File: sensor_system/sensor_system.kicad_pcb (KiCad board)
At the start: 2 copper layers, 52 parts, among them J1 Magnetic connector, J2 Solar_panels, Q1 SBC817, Q2 MJD45H11, SW1 SW_DPDT_x2, U1 TLC555xD, U2 XC6206PxxxMR, U3 MCP73833, U4 module_bme280_alt, U5 ESP32-DEVKIT-V1, U7 TPS63002

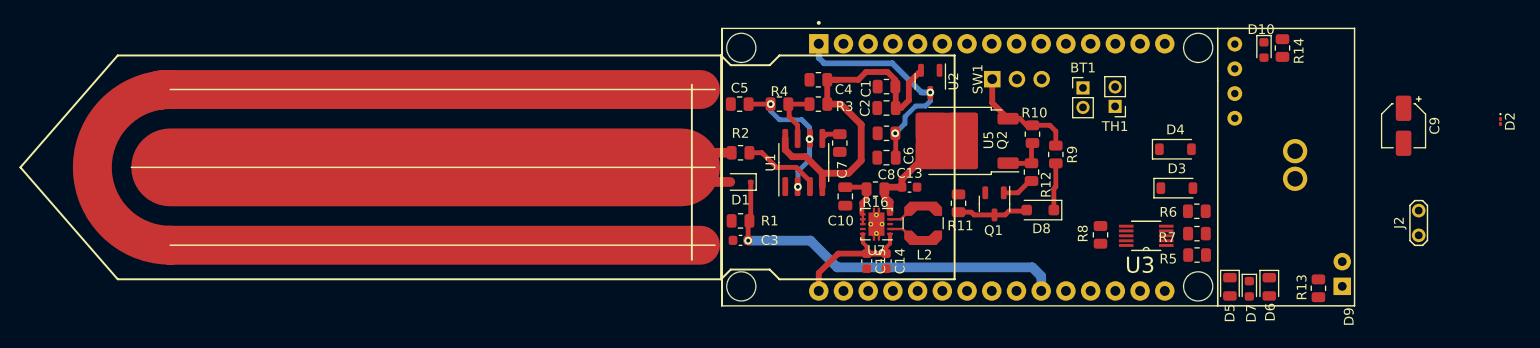
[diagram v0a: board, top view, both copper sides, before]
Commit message: Board V1 with one mistake
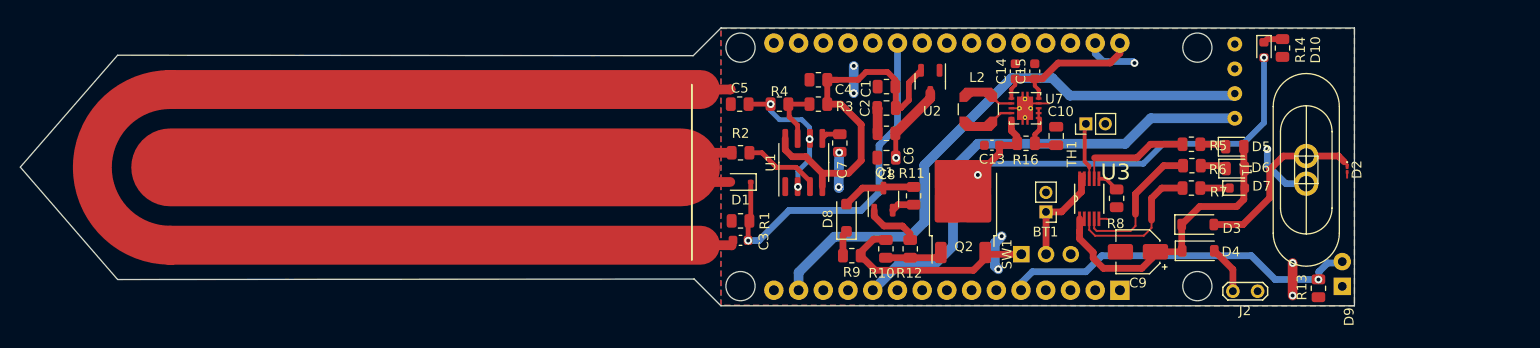
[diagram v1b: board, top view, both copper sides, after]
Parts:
- J1: moved to F.Cu
- U5: moved to B.Cu
- moved C9 30.2 mm to (137.4, 47.0), turned to 180 degrees
- moved C15 26.1 mm to (126.8, 28.4), turned to 90 degrees
- moved C14 23.6 mm to (124.8, 28.4), turned to 90 degrees
- moved R9 23.4 mm to (108.0, 47.4), turned to 180 degrees
- moved C10 22.5 mm to (129.1, 35.1), turned to 90 degrees
- moved D8 19.9 mm to (107.5, 43.5), turned to 90 degrees
- moved U7 19.4 mm to (125.8, 32.2), turned to 0 degrees
- moved R10 19.1 mm to (111.5, 46.7)
- moved SW1 18.2 mm to (125.5, 47.2)
- moved J2 17.5 mm to (149.8, 51.0), turned to 180 degrees
- moved D2 16.5 mm to (158.9, 38.5)
- moved R16 16.2 mm to (126.0, 35.9), turned to 0 degrees
- moved R12 14.7 mm to (114.0, 46.7), turned to 90 degrees
- moved D5 14.4 mm to (147.4, 36.2), turned to 0 degrees
- moved BT1 13.3 mm to (128.0, 42.9), turned to 180 degrees
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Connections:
- BT1 pad 2: GNDREF -> Earth
- C10 pad 2: GNDREF -> Earth
- C13 pad 2: GNDREF -> Earth
- C14 pad 2: GNDREF -> Earth
- C15 pad 2: GNDREF -> Earth
- C9 pad 2: GNDREF -> Earth
- D2 pad 2: GNDREF -> Earth
- J1 pad 1: GNDREF -> Earth
- J2 pad 1: GNDREF -> Earth
- Q1 pad 2: GNDREF -> Earth
- R11 pad 2: GNDREF -> Earth
- R14 pad 1: GNDREF -> Earth
- R8 pad 1: GNDREF -> Earth
- TH1 pad 2: GNDREF -> Earth
- U3 pad 5: GNDREF -> Earth
- U5 pad 19: Net-(D9-A) -> unconnected-(U5-D34-Pad19)
- U5 pad 5: unconnected-(U5-D4-Pad5) -> Net-(D9-A)
- U7 pad 11: GNDREF -> Earth
- U7 pad 3: GNDREF -> Earth
- U7 pad 9: GNDREF -> Earth
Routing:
- net Earth: track 0.00 -> 148.2 mm, vias 0 -> 8
- net (no net): track 109.1 -> 0.00 mm
- net SCL: track 0.00 -> 59.2 mm
- net SDA: track 0.00 -> 49.2 mm
- net Net-(D10-A): track 8.68 -> 47.4 mm, vias 0 -> 2
- net Net-(D9-A): track 0.00 -> 37.2 mm, vias 0 -> 1
- net Net-(D3-K): track 0.00 -> 31.0 mm
- net Net-(D2-A1): track 0.00 -> 18.9 mm
- net Net-(U3-STAT2): track 0.00 -> 14.9 mm
- net Net-(U3-STAT1): track 0.00 -> 14.8 mm
- net 3V3: track 24.2 -> 12.0 mm, vias 2 -> 3
- net Net-(U3-PG): track 0.00 -> 11.8 mm
- net Net-(BT1-+): track 0.00 -> 11.3 mm
- net Net-(Q2-E): track 12.2 -> 21.4 mm
- net Net-(U3-THERM): track 0.00 -> 6.11 mm
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- added copper zone on B.Cu, net 3V3
- added copper zone on F.Cu, net Earth
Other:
- board outline added: 137.1 x 28.5 mm
